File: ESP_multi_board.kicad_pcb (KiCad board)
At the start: 2 copper layers, 100 x 50 mm, 47 parts, among them IC101 L298, P101 CONN_01X02, P102 CONN_01X06, P103 CONN_01X02, P104 CONN_01X06, P105 CONN_01X06, P106 CONN_01X03, P107 CONN_I2C_MPU6050, P108 CONN_PINES_DIG, P109 CONN_01X04, SW101 SW_PUSH_SMALL, SW102 SWITCH_INV, U1 LD1117S33TR, U102 ESP-12, U103 MAX11605EEE+, U104 MCP23008

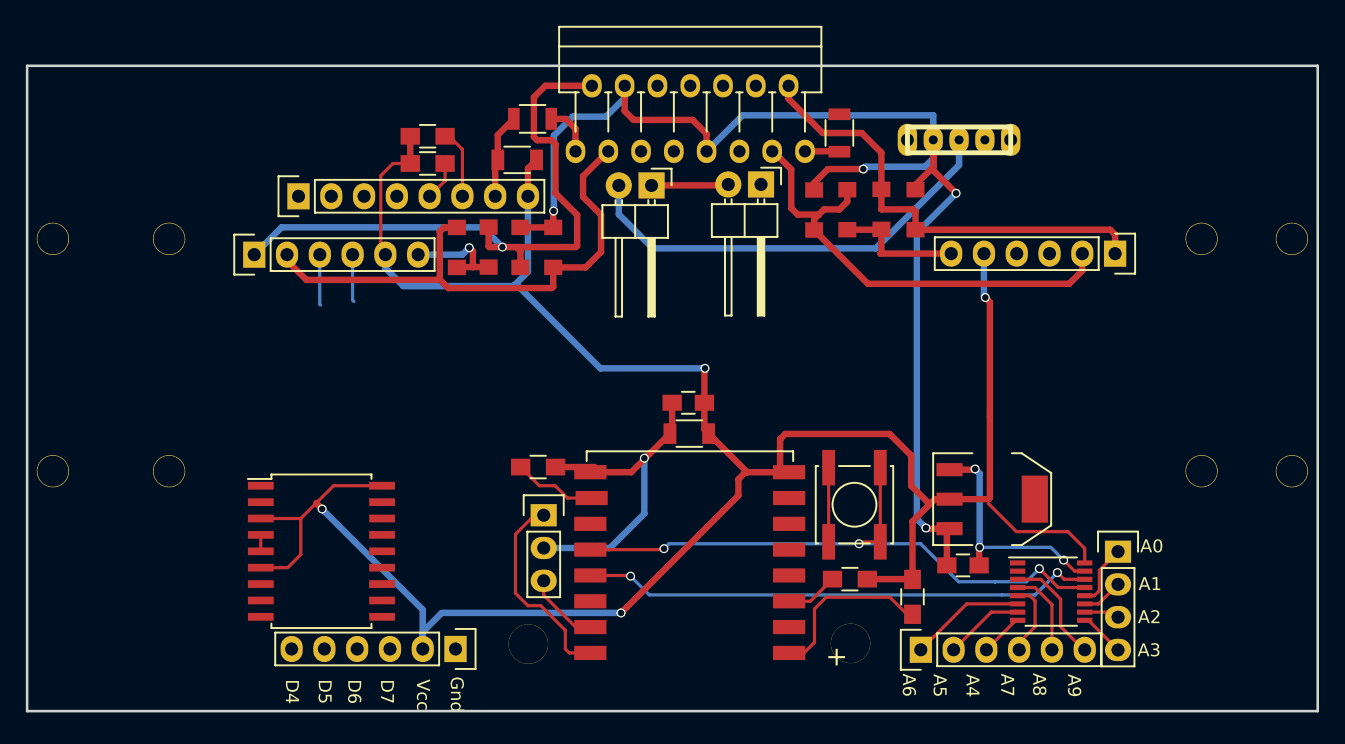
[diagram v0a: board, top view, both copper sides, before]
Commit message: Finalizado posible layout
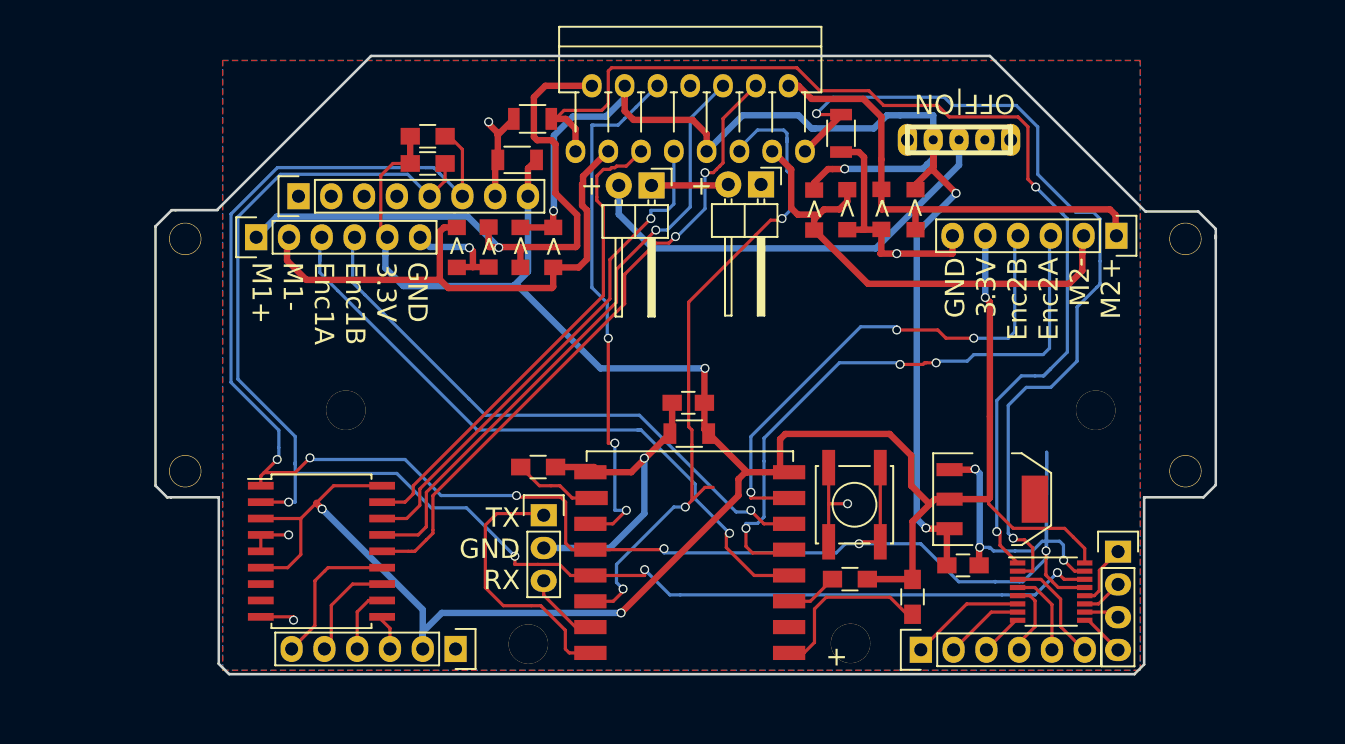
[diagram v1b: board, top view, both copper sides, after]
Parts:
- removed drill1, drill12, drill13, drill2: 1pin, Connect:1pin
- added drill8: 1pin, Connect:1pin, F.Cu at (108.7, 89.4)
- added drill8: 1pin, Connect:1pin, F.Cu at (166.8, 89.4)
- moved P104 1.39 mm to (168.4, 75.9)
- moved P102 1.35 mm to (101.8, 76.0)
- moved drill11 1.25 mm to (97.2, 77.2)
- moved drill14 1.25 mm to (97.2, 93.0)
- moved drill3 1.25 mm to (173.8, 93.0)
- moved drill4 1.25 mm to (173.8, 77.2)
- moved R107 0.13 mm to (147.1, 67.9), turned to 270 degrees
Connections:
- U104 pad 10: M1_A -> Net-(P108-Pad3)
- U104 pad 11: M1_B -> Net-(P108-Pad4)
- U104 pad 12: M2_A -> Net-(P108-Pad5)
- U104 pad 13: M2_B -> Net-(P108-Pad6)
- U104 pad 14: Net-(P108-Pad6) -> M2_B
- U104 pad 15: Net-(P108-Pad5) -> M2_A
- U104 pad 16: Net-(P108-Pad4) -> M1_B
- U104 pad 17: Net-(P108-Pad3) -> M1_A
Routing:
- net SCL: track 52.9 -> 147.0 mm, vias 3 -> 6
- net CURRENT1: track 3.95 -> 85.8 mm, vias 0 -> 2
- net SDA: track 42.2 -> 113.8 mm, vias 2 -> 4
- net CURRENT2: track 2.68 -> 68.4 mm, vias 0 -> 2
- net EN2: track 0.00 -> 51.7 mm, vias 0 -> 3
- net M2_B: track 0.00 -> 50.6 mm, vias 0 -> 2
- net M2_A: track 0.00 -> 47.9 mm, vias 0 -> 1
- net ENC2_A: track 0.00 -> 47.7 mm, vias 0 -> 3
- net ENC1_A: track 3.93 -> 50.9 mm, vias 0 -> 1
- net ENC1_B: track 3.67 -> 44.7 mm, vias 0 -> 1
- net EN1: track 0.00 -> 40.7 mm, vias 0 -> 3
- net M1_B: track 0.00 -> 39.7 mm, vias 0 -> 1
- net ENC2_B: track 0.00 -> 39.4 mm, vias 0 -> 3
- net M1_A: track 0.00 -> 37.8 mm
- net GND: track 76.5 -> 95.0 mm, vias 5 -> 10
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- added copper zone on B.Cu, net GND
- added copper zone on F.Cu, net GND
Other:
- board size 100 x 50 mm -> 82.1 x 47.9 mm
- net class Default: trace_width 0.25 -> 0.5
- board text added: "+ -"
- board text added: "3.3V"
- board text added: ">"
- board text added: "GND"
- board text added: "GND 3.3V Enc1B Enc1A M1- M1+"
- board text added: "GND 3.3V Enc2B Enc2A M2- M2+"
- board text added: "GND 3.3V GP0 GP1 GP2 GP3"
- board text added: "OFF|ON"
- board text added: "SCL"
- board text added: "SDA"
- board text added: "TX GND RX"
- board text removed: "D4"
- board text removed: "D5"
- board text removed: "D6"
- board text removed: "D7"
- board text removed: "Gnd"
- board text removed: "Vcc"
